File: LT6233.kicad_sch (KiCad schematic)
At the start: 15 parts, among them U3001 LT6233CS6TRMPBF, U3002 PBSS4230T

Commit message: fields
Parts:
- C3001, C3005: gfootprint 2917 -> (none)
- C3002, C3008: gfootprint 1206 -> (none)
- C3003, C3006, C3007, R3001, R3002, R3003: gfootprint 0603 -> (none)
- C3004: gfootprint 0402 -> (none)
- FB3001, FB3002: gfootprint 0805 -> (none)
- U3001: Availability In Stock -> (none); COPYRIGHT Copyright C 2016 Accelerated Designs. All rights reserved -> (none); Check_prices https://www.snapeda.com/parts/LT6233CS6%23TRMPBF/Analog+Dev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 -> (none); DIGIKEY_PART_NUMBER LT6233CS6#TRMPBFTRND -> (none); Description_1 General Purpose Amplifier 1 Circuit Rail-to-Rail TSOT-23-6 -> (none); MANUFACTURER_PART_NUMBER LT6233CS6#TRMPBF -> (none); MF Analog Devices -> (none); MP LT6233CS6#TRMPBF -> (none); Package SOT-23-6 Linear Technology -> (none); Price None -> (none); Purchase-URL https://www.snapeda.com/api/url_track_click_mouser/?unipart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 -> (none); SnapEDA_Link https://www.snapeda.com/parts/LT6233CS6%23TRMPBF/Analog+Dev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 -> (none); VENDOR Linear Technology -> (none)

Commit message: vendor info
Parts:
- C3001, C3005: footprint 001_download:CAP_EEF_CD_PAN -> 001_download:CAP_EEF_CD_PAN_GH; Vendor (none) -> digikey:PCE3168CT-ND
- C3002, C3008: Vendor (none) -> digikey:490-5528-1-ND
- C3003, C3006, C3007: Vendor (none) -> digikey:490-3897-1-ND
- C3004: Vendor (none) -> digikey:490-1318-1-ND
- FB3001, FB3002: Vendor (none) -> digikey:732-1620-1-ND
- R3001: Vendor (none) -> digikey:311-4.42KHRCT-ND
- R3002: Vendor (none) -> digikey:311-11.5KHRCT-ND
- R3003: Vendor (none) -> digikey:RR08P200DCT-ND
- U3001: Vendor (none) -> digikey:LT6233CS6#TRMPBFCT-ND
- U3002: Vendor (none) -> digikey:568-4155-1-ND
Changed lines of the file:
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@@
+			)
+		)
+		(property "Vendor" "digikey:490-5528-1-ND"
+			(at 464.82 0 0)
+			(effects
+				(font
+					(size 1.27 1.27)
+				)
+				(hide yes)
 			)
 		)
@@
 			)
 		)
+		(property "Vendor" "digikey:732-1620-1-ND"
+			(at 111.76 -111.76 0)
+			(effects
+				(font
+					(size 1.27 1.27)
+				)
+				(hide yes)
+			)
+		)
 		(pin "1"
 		)
@@
 			)
 		)
+		(property "Vendor" "digikey:490-3897-1-ND"
+			(at 0 0 0)
+			(effects
+				(font
+					(size 1.27 1.27)
+				)
+				(hide yes)
+			)
+		)
 		(pin "2"
 		)
@@
 			)
 		)
+		(property "Vendor" "digikey:LT6233CS6#TRMPBFCT-ND"
+			(at 0 198.12 0)
+			(effects
+				(font
+					(size 1.27 1.27)
+				)
+				(hide yes)
+			)
+		)
 		(pin "2"
 		)
@@
 			)
 		)
+		(property "Vendor" "digikey:732-1620-1-ND"
+			(at 25.4 -25.4 0)
+			(effects
+				(font
+					(size 1.27 1.27)
+				)
+				(hide yes)
+			)
+		)
 		(pin "1"
 		)
@@
 			)
 		)
-		(property "Footprint" "001_download:CAP_EEF_CD_PAN"
+		(property "Footprint" "001_download:CAP_EEF_CD_PAN_GH"
 			(at 144.4752 123.19 0)
 			(effects
@@
 		(property "Description" "Unpolarized capacitor"
 			(at 143.51 119.38 0)
+			(effects
+				(font
+					(size 1.27 1.27)
+				)
+				(hide yes)
+			)
+		)
+		(property "Vendor" "digikey:PCE3168CT-ND"
+			(at 0 238.76 0)
 			(effects
 				(font
@@
 			)
 		)
+		(property "Vendor" "digikey:490-1318-1-ND"
+			(at 256.54 0 0)
+			(effects
+				(font
+					(size 1.27 1.27)
+				)
+				(hide yes)
+			)
+		)
 		(pin "2"
 		)
@@
 			)
 		)
+		(property "Vendor" "digikey:490-5528-1-ND"
+			(at 205.74 0 0)
+			(effects
+				(font
+					(size 1.27 1.27)
+				)
+				(hide yes)
+			)
+		)
 		(pin "2"
 		)
@@
 		(property "Description" "Unpolarized capacitor"
 			(at 219.71 88.9 0)
+			(effects
+				(font
+					(size 1.27 1.27)
+				)
+				(hide yes)
+			)
+		)
+		(property "Vendor" "digikey:490-3897-1-ND"
+			(at 439.42 0 0)
 			(effects
 				(font
@@
 			)
 		)
+		(property "Vendor" "digikey:311-11.5KHRCT-ND"
+			(at 106.68 0 0)
+			(effects
+				(font
+					(size 1.27 1.27)
+				)
+				(hide yes)
+			)
+		)
 		(pin "1"
 		)
@@
 		(property "Description" "Unpolarized capacitor"
 			(at 156.21 119.38 0)
+			(effects
+				(font
+					(size 1.27 1.27)
+				)
+				(hide yes)
+			)
+		)
+		(property "Vendor" "digikey:490-3897-1-ND"
+			(at 312.42 0 0)
 			(effects
 				(font
@@
 			)
 		)
+		(property "Vendor" "digikey:RR08P200DCT-ND"
+			(at 248.92 248.92 0)
+			(effects
+				(font
+					(size 1.27 1.27)
+				)
+				(hide yes)
+			)
+		)
 		(pin "1"
 		)
@@
 			)
 		)
-		(property "Footprint" "001_download:CAP_EEF_CD_PAN"
+		(property "Footprint" "001_download:CAP_EEF_CD_PAN_GH"
 			(at 43.4848 113.03 0)
 			(effects
@@
 		(property "Description" "Unpolarized capacitor"
 			(at 44.45 109.22 0)
+			(effects
+				(font
+					(size 1.27 1.27)
+				)
+				(hide yes)
+			)
+		)
+		(property "Vendor" "digikey:PCE3168CT-ND"
+			(at 88.9 218.44 0)
 			(effects
 				(font
@@
 			)
 		)
+		(property "Vendor" "digikey:311-4.42KHRCT-ND"
+			(at 106.68 0 0)
+			(effects
+				(font
+					(size 1.27 1.27)
+				)
+				(hide yes)
+			)
+		)
 		(pin "1"
 		)
@@
 			(effects
 				(font
+					(size 1.27 1.27)
+				)
+				(hide yes)
+			)
+		)
+		(property "Vendor" "digikey:568-4155-1-ND"
+			(at 0 170.18 0)
+			(effects
+				(font

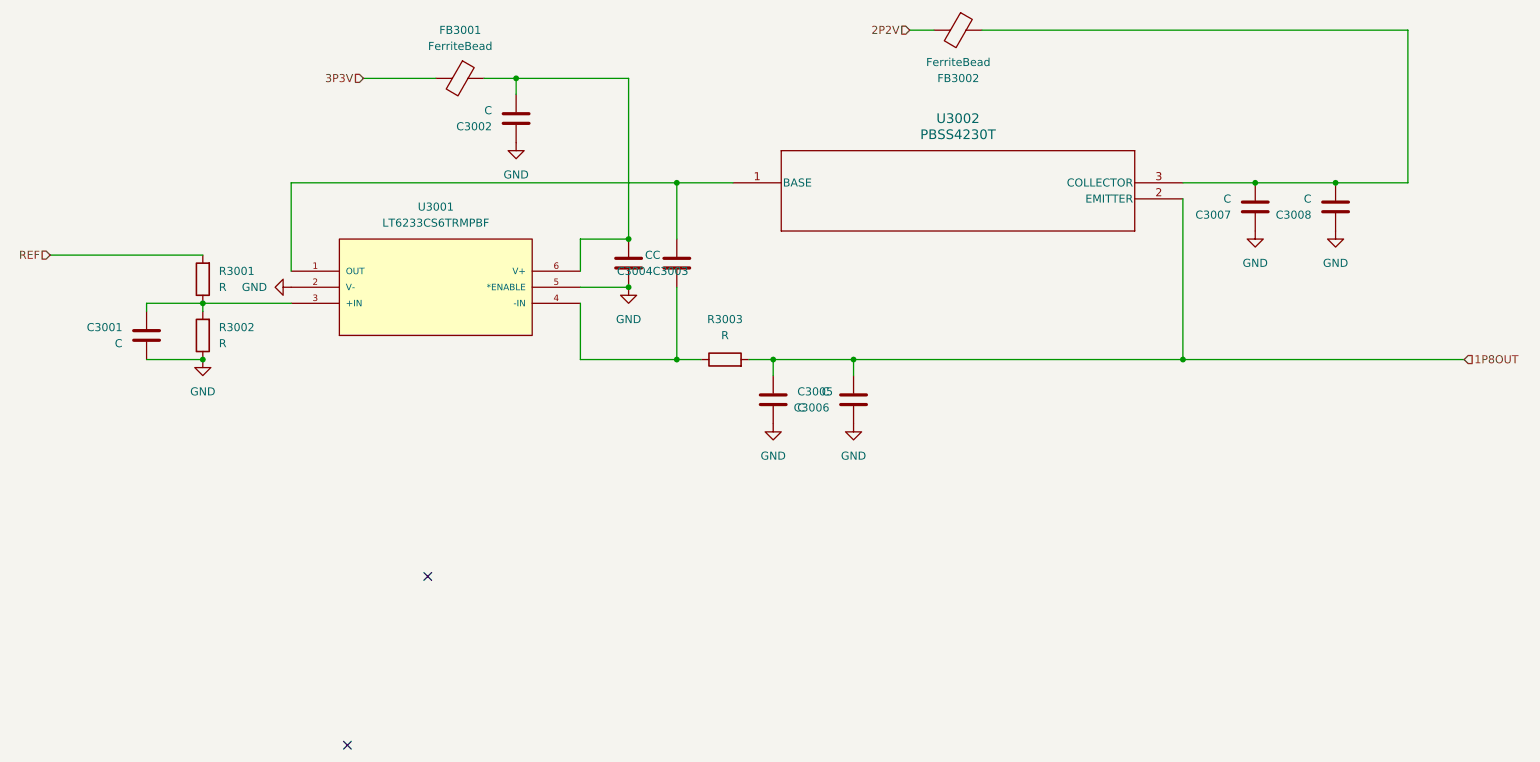
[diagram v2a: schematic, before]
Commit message: update value
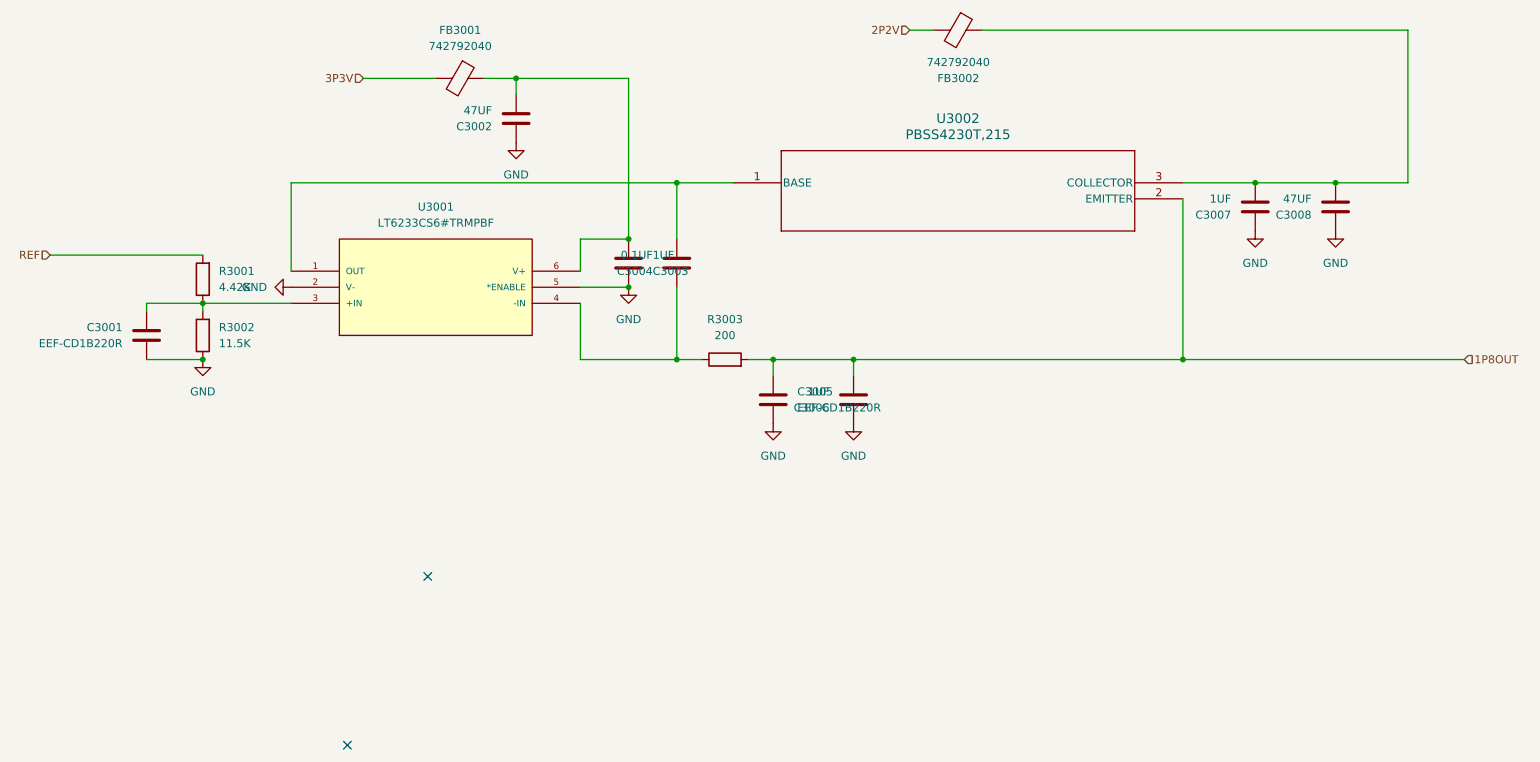
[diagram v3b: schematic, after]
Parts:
- C3001, C3005: value C -> EEF-CD1B220R
- C3002, C3008: value C -> 47UF
- C3003, C3006, C3007: value C -> 1UF
- C3004: value C -> 0.1UF
- FB3001, FB3002: value FerriteBead -> 742792040
- R3001: value R -> 4.42K
- R3002: value R -> 11.5K
- R3003: value R -> 200
- U3001: value LT6233CS6TRMPBF -> LT6233CS6#TRMPBF
- U3002: value PBSS4230T -> PBSS4230T,215
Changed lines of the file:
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@@
 			)
 		)
-		(property "Value" "C"
+		(property "Value" "47UF"
 			(at 228.6 87.6301 0)
 			(effects
@@
 			)
 		)
-		(property "Value" "FerriteBead"
+		(property "Value" "742792040"
 			(at 172.7708 66.04 90)
 			(effects
@@
 			)
 		)
-		(property "Value" "C"
+		(property "Value" "1UF"
 			(at 124.46 96.5201 0)
 			(effects
@@
 			)
 		)
-		(property "Value" "LT6233CS6TRMPBF"
+		(property "Value" "LT6233CS6#TRMPBF"
 			(at 90.17 91.44 0)
 			(effects
@@
 			)
 		)
-		(property "Value" "FerriteBead"
+		(property "Value" "742792040"
 			(at 94.0308 63.5 90)
 			(effects
@@
 			)
 		)
-		(property "Value" "C"
+		(property "Value" "EEF-CD1B220R"
 			(at 147.32 120.6499 0)
 			(effects
@@
 			)
 		)
-		(property "Value" "C"
+		(property "Value" "0.1UF"
 			(at 124.46 96.5201 0)
 			(effects
@@
 			)
 		)
-		(property "Value" "C"
+		(property "Value" "47UF"
 			(at 99.06 73.6601 0)
 			(effects
@@
 			)
 		)
-		(property "Value" "C"
+		(property "Value" "1UF"
 			(at 215.9 87.6301 0)
 			(effects
@@
 			)
 		)
-		(property "Value" "R"
+		(property "Value" "11.5K"
 			(at 55.88 110.4899 0)
 			(effects
@@
 			)
 		)
-		(property "Value" "C"
+		(property "Value" "1UF"
 			(at 152.4 118.1101 0)
 			(effects
@@
 			)
 		)
-		(property "Value" "R"
+		(property "Value" "200"
 			(at 135.89 109.22 90)
 			(effects
@@
 			)
 		)
-		(property "Value" "C"
+		(property "Value" "EEF-CD1B220R"
 			(at 40.64 110.4899 0)
 			(effects
@@
 			)
 		)
-		(property "Value" "R"
+		(property "Value" "4.42K"
 			(at 55.88 101.5999 0)
 			(effects
@@
 			)
 		)
-		(property "Value" "PBSS4230T"
+		(property "Value" "PBSS4230T,215"
 			(at 172.72 77.47 0)
 			(effects

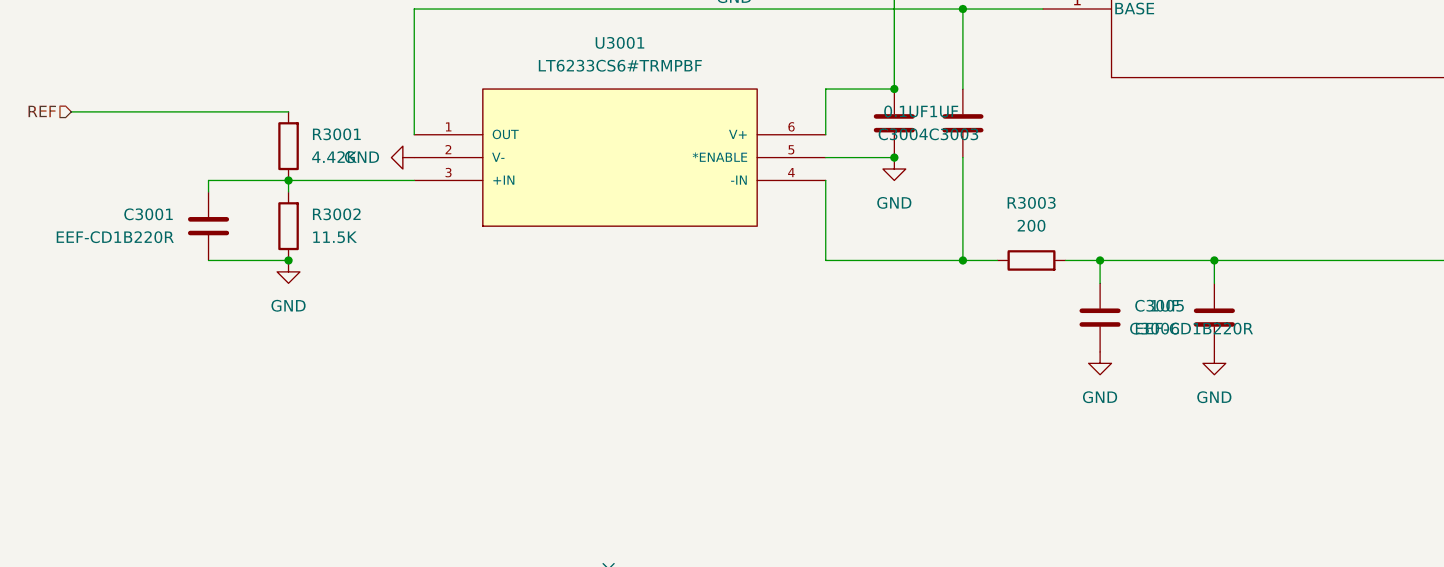
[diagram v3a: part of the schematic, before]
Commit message: value
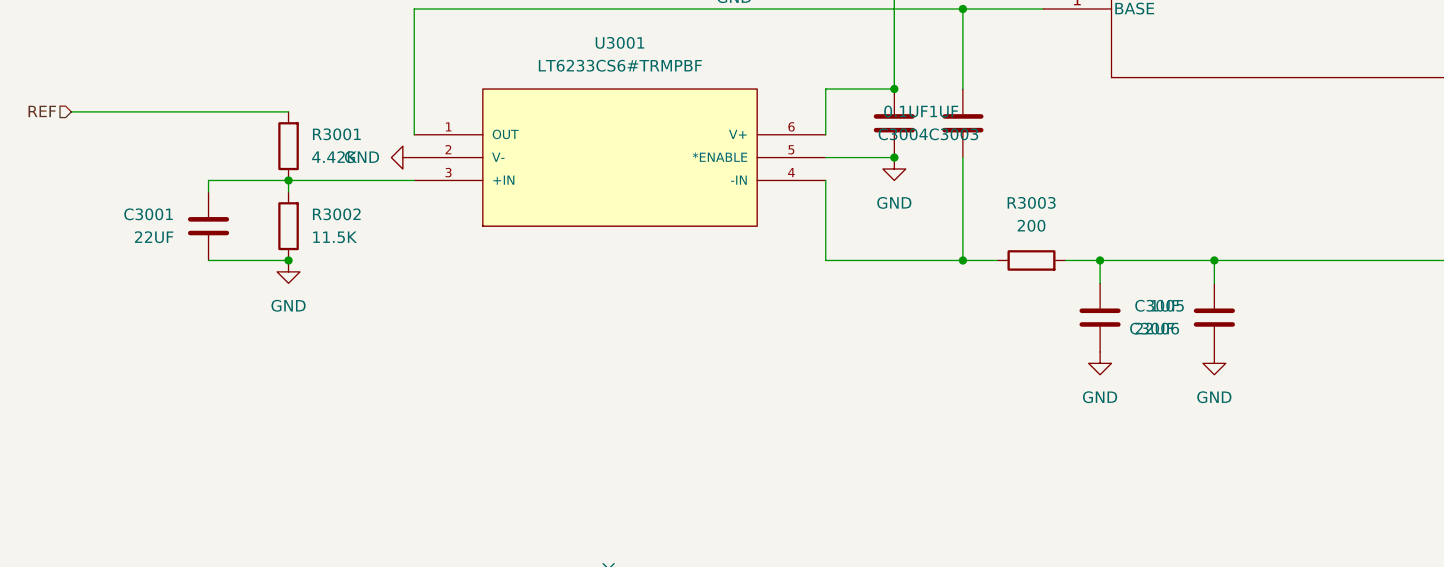
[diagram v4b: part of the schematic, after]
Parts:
- C3001, C3005: value EEF-CD1B220R -> 22UF
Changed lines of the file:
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@@
 			)
 		)
-		(property "Value" "EEF-CD1B220R"
+		(property "Value" "22UF"
 			(at 147.32 120.6499 0)
 			(effects
@@
 			)
 		)
-		(property "Description" "Unpolarized capacitor"
+		(property "Description" "Al-Poly"
 			(at 143.51 119.38 0)
 			(effects
@@
 			)
 		)
-		(property "Value" "EEF-CD1B220R"
+		(property "Value" "22UF"
 			(at 40.64 110.4899 0)
 			(effects
@@
 			)
 		)
-		(property "Description" "Unpolarized capacitor"
+		(property "Description" "Al-Poly"
 			(at 44.45 109.22 0)
 			(effects

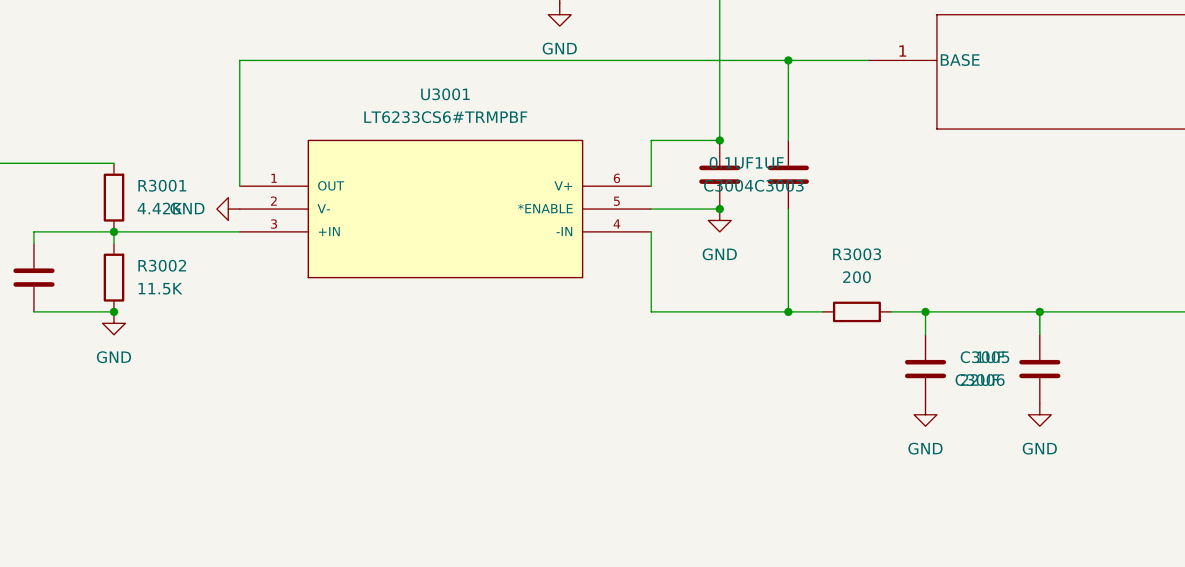
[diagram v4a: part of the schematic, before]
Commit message: lots small updates
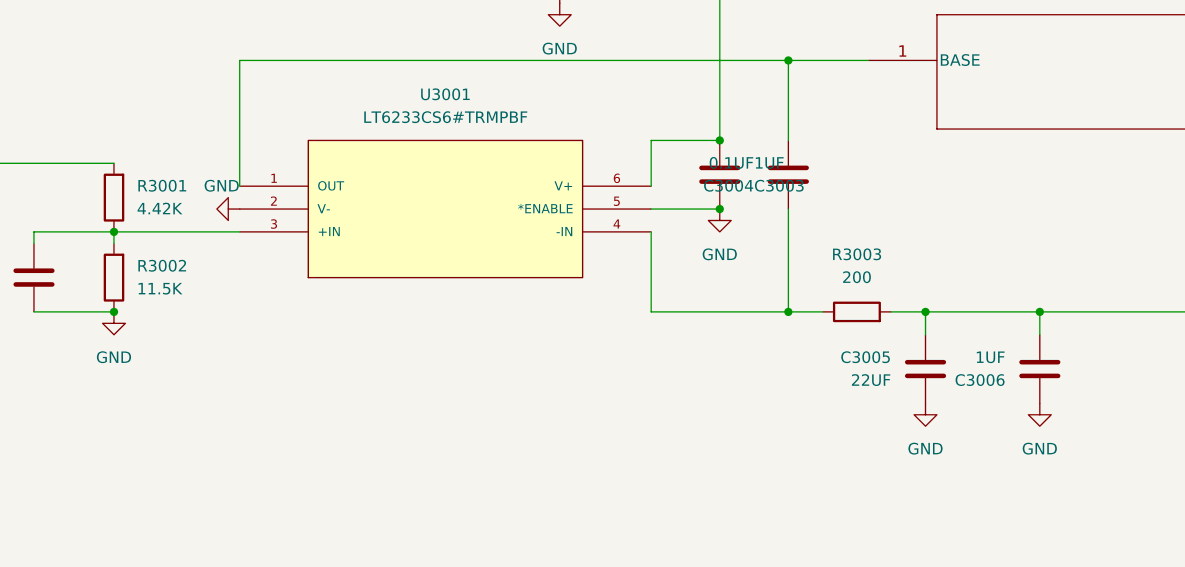
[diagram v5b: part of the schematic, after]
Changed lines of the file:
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@@
 		(lib_id "Device:C")
 		(at 143.51 119.38 0)
+		(mirror y)
 		(unit 1)
 		(exclude_from_sim no)
@@
 		(dnp no)
 		(property "Reference" "C3005"
-			(at 147.32 118.1099 0)
+			(at 139.7 118.1099 0)
 			(effects
 				(font
@@
 		)
 		(property "Value" "22UF"
-			(at 147.32 120.6499 0)
+			(at 139.7 120.6499 0)
 			(effects
 				(font
@@
 		)
 		(property "Footprint" "001_download:CAP_EEF_CD_PAN_GH"
-			(at 144.4752 123.19 0)
+			(at 142.5448 123.19 0)
 			(effects
 				(font
@@
 		)
 		(property "Vendor" "digikey:PCE3168CT-ND"
-			(at 0 238.76 0)
+			(at 287.02 238.76 0)
 			(effects
 				(font
@@
 		(on_board yes)
 		(dnp no)
-		(fields_autoplaced yes)
 		(property "Reference" "#PWR03008"
 			(at 60.96 101.6 0)
@@
 		)
 		(property "Value" "GND"
-			(at 63.5 101.5999 90)
-			(effects
-				(font
+			(at 67.31 99.06 90)
+			(effects
+				(font
